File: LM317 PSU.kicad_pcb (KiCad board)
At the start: 2 copper layers, 100 x 80 mm, 58 parts, among them J1 4MM Red female, J2 4MM Black female, J3 Barrel_Jack_MountingPin, Q1 2N2222, SW1 SW_Push_SPDT, U1 NA555, U2 TL061, U3 LM358, U4 LM317_3PinPackage, U5 LM358

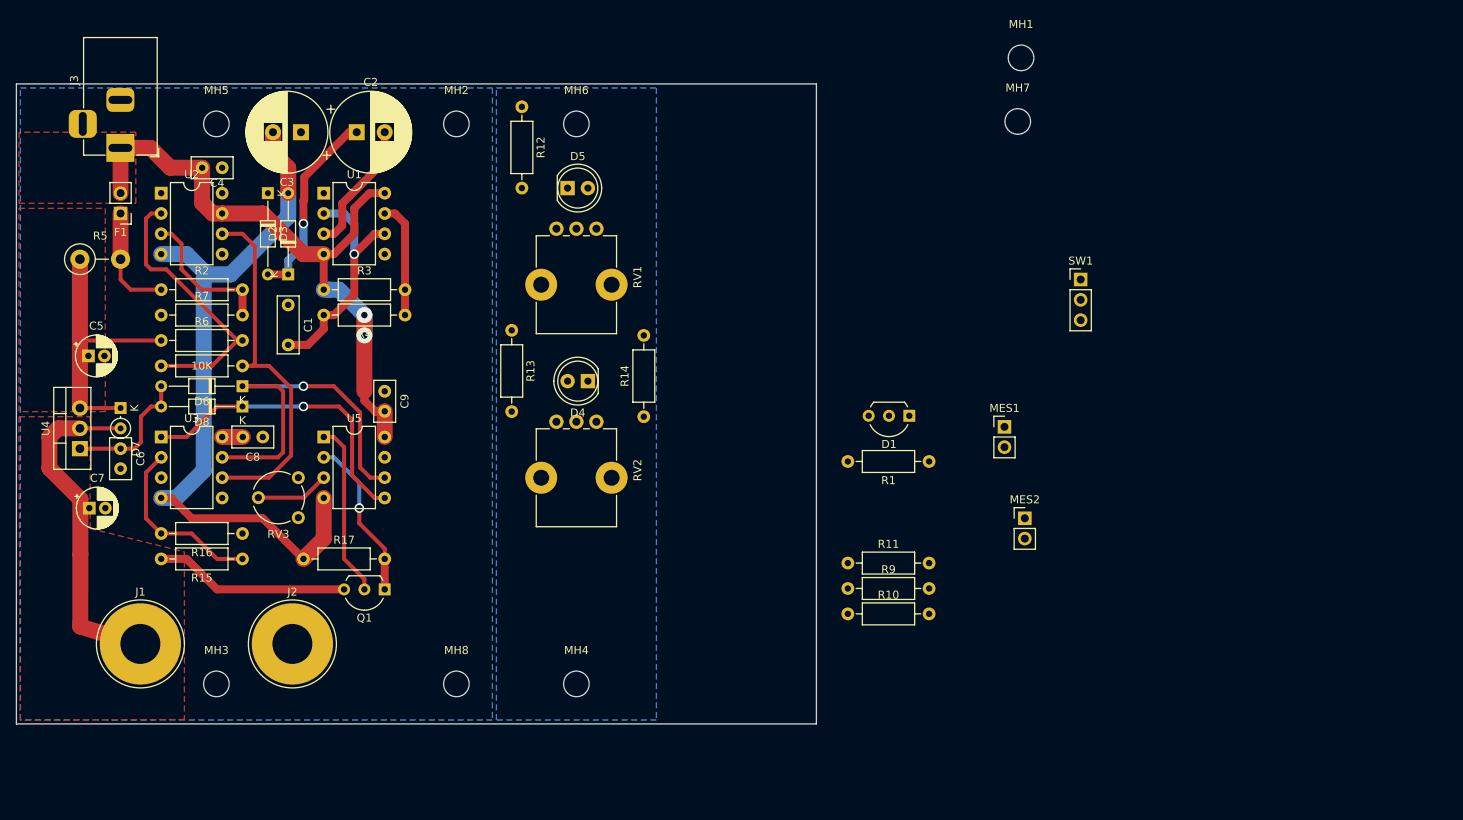
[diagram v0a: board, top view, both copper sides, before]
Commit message: Rev 1 mostly complete
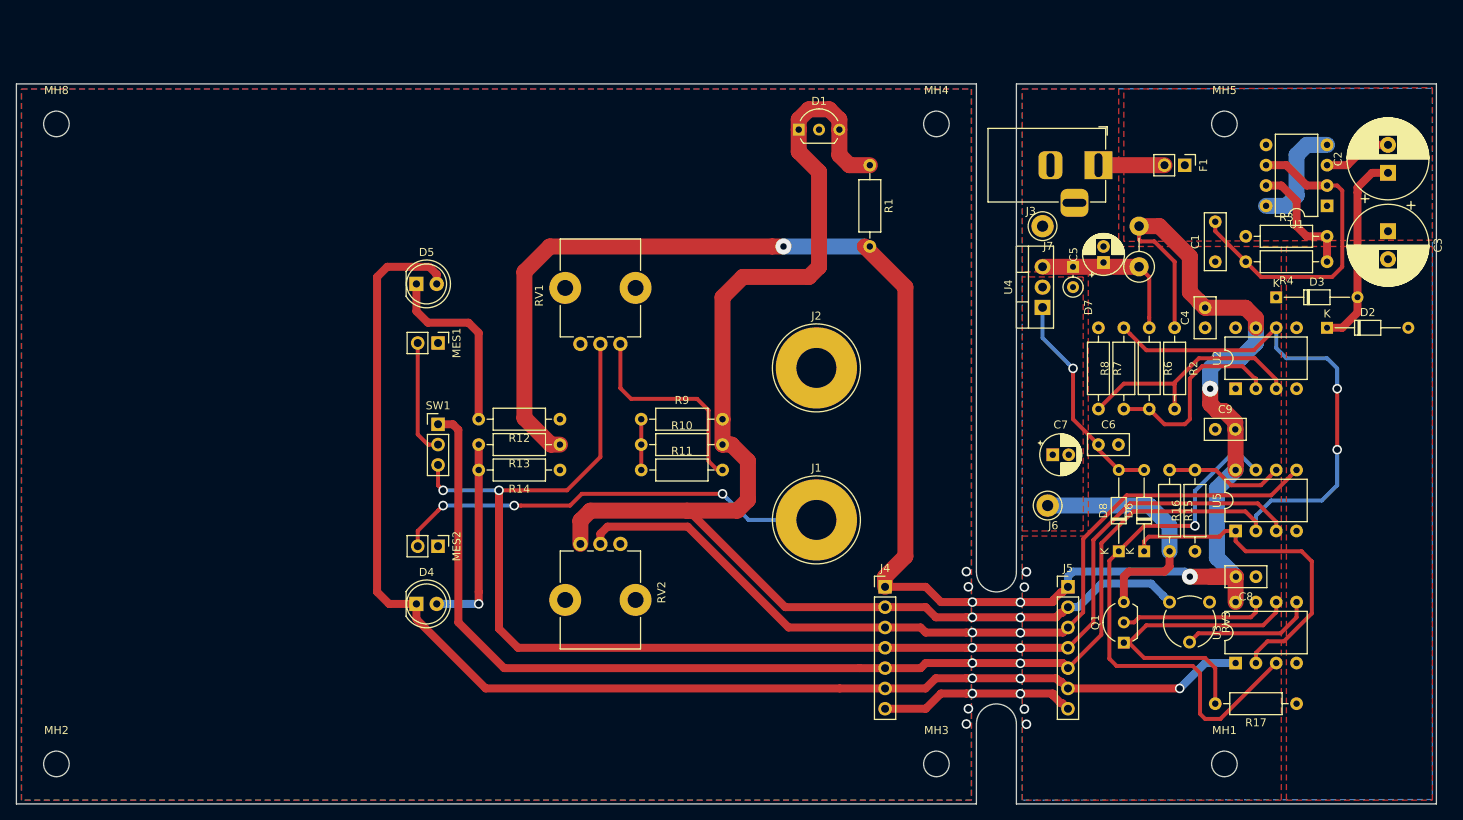
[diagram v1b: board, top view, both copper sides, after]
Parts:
- removed MH6, MH7: MountingHole, MountingHole:MountingHole_3.2mm_M3
- added J4: Conn_01x07_Male, Connector_PinHeader_2.54mm:PinHeader_1x07_P2.54mm_Vertical, F.Cu at (128.6, 82.9)
- added J5: Conn_01x07_Female, Connector_PinHeader_2.54mm:PinHeader_1x07_P2.54mm_Vertical, F.Cu at (151.4, 82.9)
- added J6: Conn_01x01_Female, TestPoint:TestPoint_Loop_D3.50mm_Drill1.4mm_Beaded, F.Cu at (148.9, 72.7)
- added J7: Conn_01x01_Female, TestPoint:TestPoint_Loop_D3.50mm_Drill1.4mm_Beaded, F.Cu at (148.3, 37.8)
- moved U3 137.2 mm to (172.4, 92.4), turned to 90 degrees
- moved U2 136.5 mm to (172.4, 58.1), turned to 90 degrees
- moved C3 136.4 mm to (191.4, 38.4), turned to 270 degrees
- moved F1 133.2 mm to (166.1, 30.2), turned to 270 degrees
- moved R5 132.4 mm to (160.3, 42.9), turned to 90 degrees
- moved D2 130.0 mm to (183.8, 50.5), turned to 0 degrees
- moved C2 129.0 mm to (191.4, 31.1), turned to 90 degrees
- moved C5 127.4 mm to (155.9, 42.3), turned to 90 degrees
- moved R2 126.8 mm to (164.8, 50.5), turned to 270 degrees
- moved D3 126.7 mm to (177.5, 46.7), turned to 0 degrees
- moved MH5 126.0 mm to (171.0, 25.0)
- moved R17 125.5 mm to (180.0, 97.5), turned to 180 degrees
- moved U1 125.4 mm to (183.8, 35.2), turned to 180 degrees
- moved C8 125.4 mm to (174.9, 81.6)
- moved C4 124.5 mm to (168.6, 50.5), turned to 90 degrees
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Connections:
- C4 pad 2: +12V -> 12V_F
- C8 pad 2: +12V -> 12V_F
- C9 pad 2: +12V -> 12V_F
- F1 pad 1: Net-(F1-Pad1) -> 12V_F
- R1 pad 2: +12V -> 12V_F
- R13 pad 1: +12V -> 12V_F
- R2 pad 1: Net-(F1-Pad1) -> 12V_F
- R3 pad 1: +12V -> 12V_F
- R5 pad 2: Net-(F1-Pad1) -> 12V_F
- U1 pad 4: +12V -> 12V_F
- U1 pad 5: (no net) -> Net-(U1-Pad5)
- U1 pad 8: +12V -> 12V_F
- U2 pad 1: (no net) -> Net-(U2-Pad1)
- U2 pad 5: (no net) -> Net-(U2-Pad5)
- U2 pad 7: +12V -> 12V_F
- U2 pad 8: (no net) -> Net-(U2-Pad8)
- U3 pad 1: /V_cmp -> LED
- U3 pad 2: Net-(R15-Pad1) -> /I_cmp
- U3 pad 3: V_SET -> /V_cmp
- U3 pad 5: I_SET -> Net-(RV3-Pad2)
- U3 pad 6: I_FB -> /I_sink_sense
- U3 pad 7: /I_cmp -> Net-(Q1-Pad2)
- U3 pad 8: +12V -> 12V_F
- U5 pad 1: Net-(Q1-Pad2) -> /I_cmp
- U5 pad 2: /I_sink_sense -> I_FB
- U5 pad 3: Net-(RV3-Pad2) -> I_SET
- U5 pad 5: /V_cmp -> V_SET
- U5 pad 6: /I_cmp -> Net-(R15-Pad1)
- U5 pad 7: LED -> /V_cmp
- U5 pad 8: +12V -> 12V_F
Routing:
- net 12V_F: track 0.00 -> 258.6 mm, vias 0 -> 5
- net I_SET: track 0.00 -> 170.0 mm, vias 0 -> 4
- net 2V5: track 0.00 -> 168.8 mm, vias 0 -> 2
- net LED: track 0.00 -> 164.7 mm, vias 0 -> 3
- net I_FB: track 45.2 -> 206.8 mm, vias 0 -> 4
- net V_SET: track 0.00 -> 107.9 mm, vias 0 -> 2
- net V-: track 92.3 -> 0.00 mm
- net +12V: track 84.8 -> 8.25 mm, vias 2 -> 0
- net /V_cmp: track 38.3 -> 69.1 mm
- net Net-(R11-Pad2): track 0.00 -> 26.3 mm
- net Net-(D4-Pad2): track 0.00 -> 25.2 mm, vias 0 -> 1
- net GNDA: track 0.00 -> 24.6 mm, vias 0 -> 2
- net Net-(D5-Pad1): track 0.00 -> 23.1 mm
- net OUTPUT: track 67.2 -> 86.2 mm, vias 0 -> 3
- net /I_sink_sense: track 20.4 -> 38.5 mm, vias 1 -> 0
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- added copper zone on F.Cu, net 12V_F
- added copper zone on F.Cu, net GNDA
- added copper zone on F.Cu, net V-
- removed copper zone on F.Cu, net +12V
- removed copper zone on F.Cu, net /REG_INP
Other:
- board size 100 x 80 mm -> 177.5 x 90 mm
- board text added: "CC"
- board text added: "CV"
- board text added: "POWER CONNECTORS"
